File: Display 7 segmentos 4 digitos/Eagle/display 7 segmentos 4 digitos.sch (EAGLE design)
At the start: 18 parts, among them T1 2N3904, T2 2N3904, T3 2N3904, T4 2N3904, U1 ARDUINOR3-BPLACE

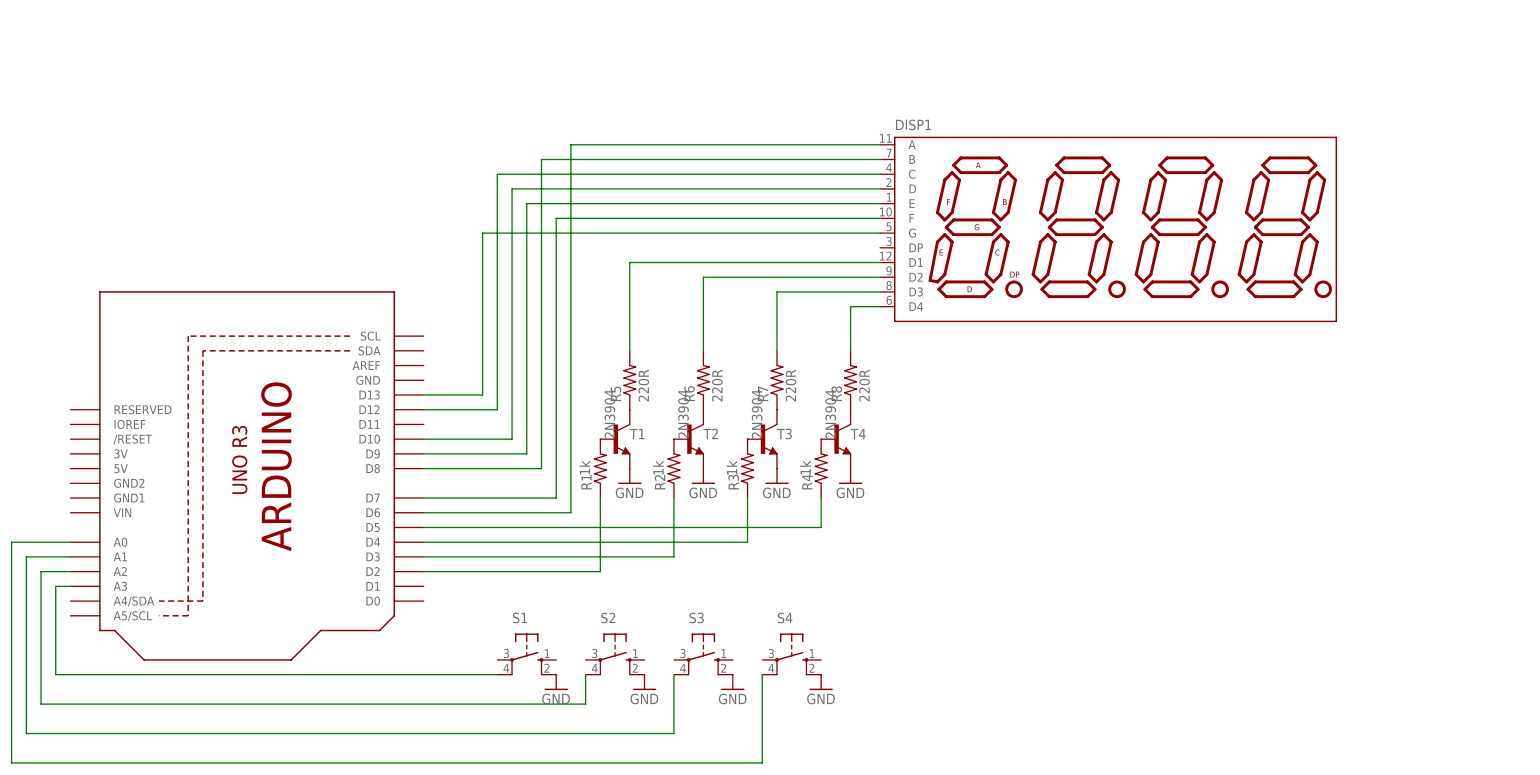
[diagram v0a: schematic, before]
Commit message: Add files via upload
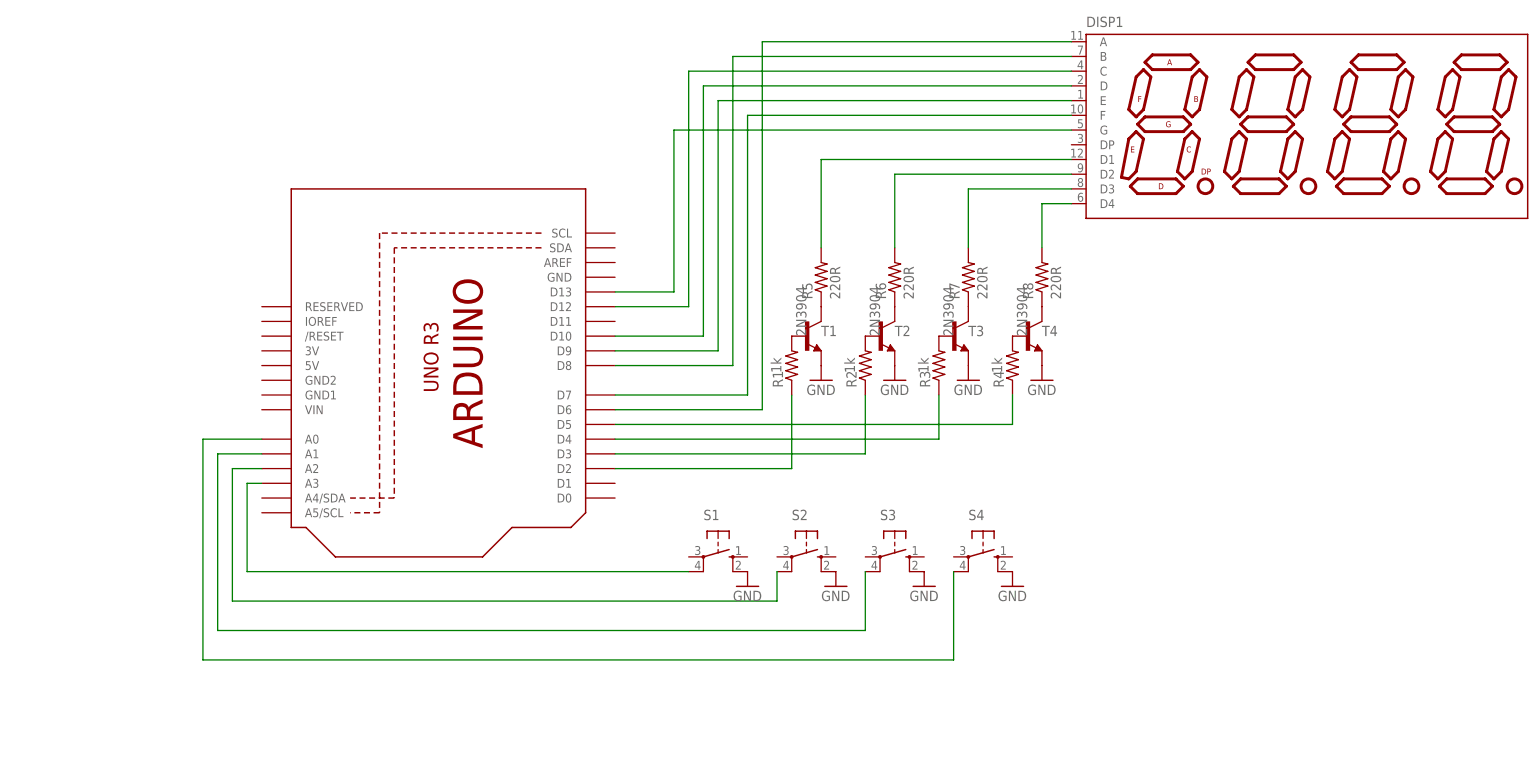
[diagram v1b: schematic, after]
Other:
- moved on the sheet: DISP1, R1, R2, R3, R4, R5, R6, R7, R8, S1, S2, S3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
